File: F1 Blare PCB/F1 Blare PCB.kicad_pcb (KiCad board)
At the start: 2 copper layers, 79 x 58 mm, 11 parts, among them J1 Conn_01x08_Pin, SW1 SW_Push, SW2 SW_Push, SW3 SW_Push, SW4 SW_Push, U1 XIAO-ESP32-C3-SMD

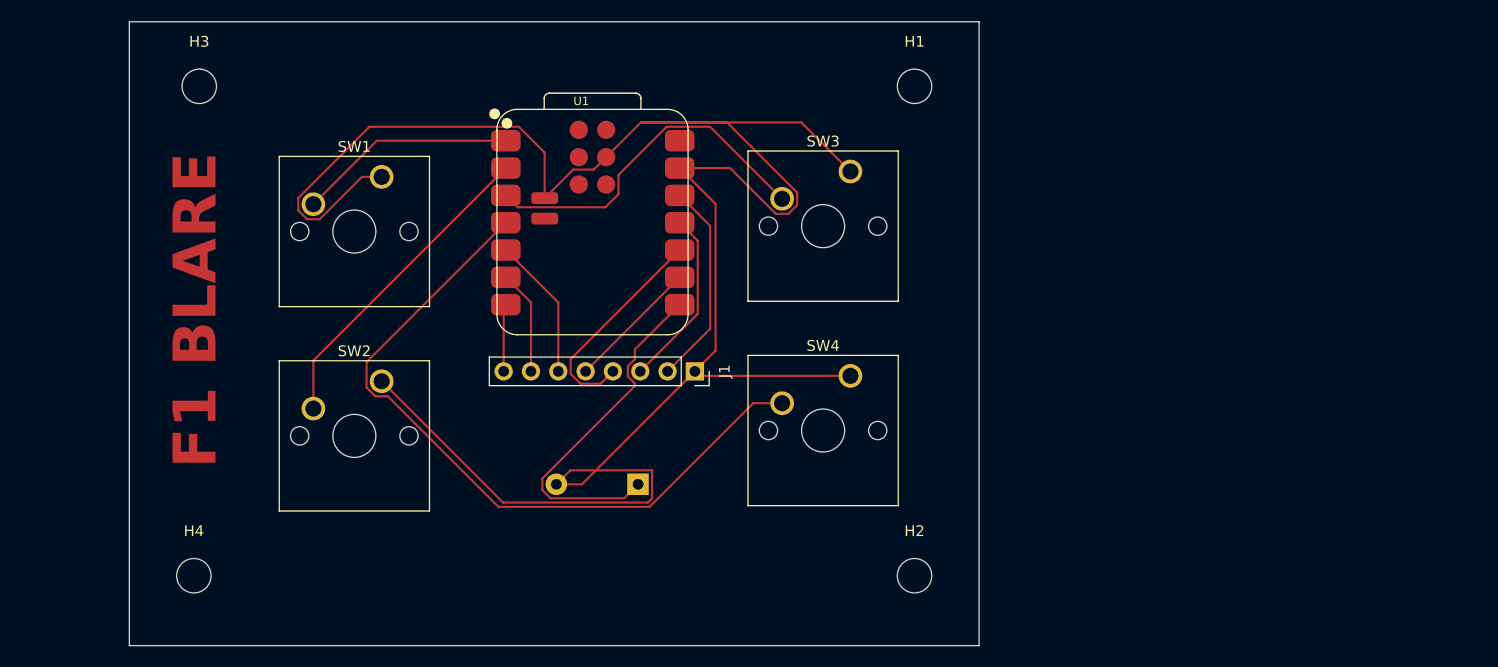
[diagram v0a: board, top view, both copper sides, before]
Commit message: PCB Finalization & CAD Design
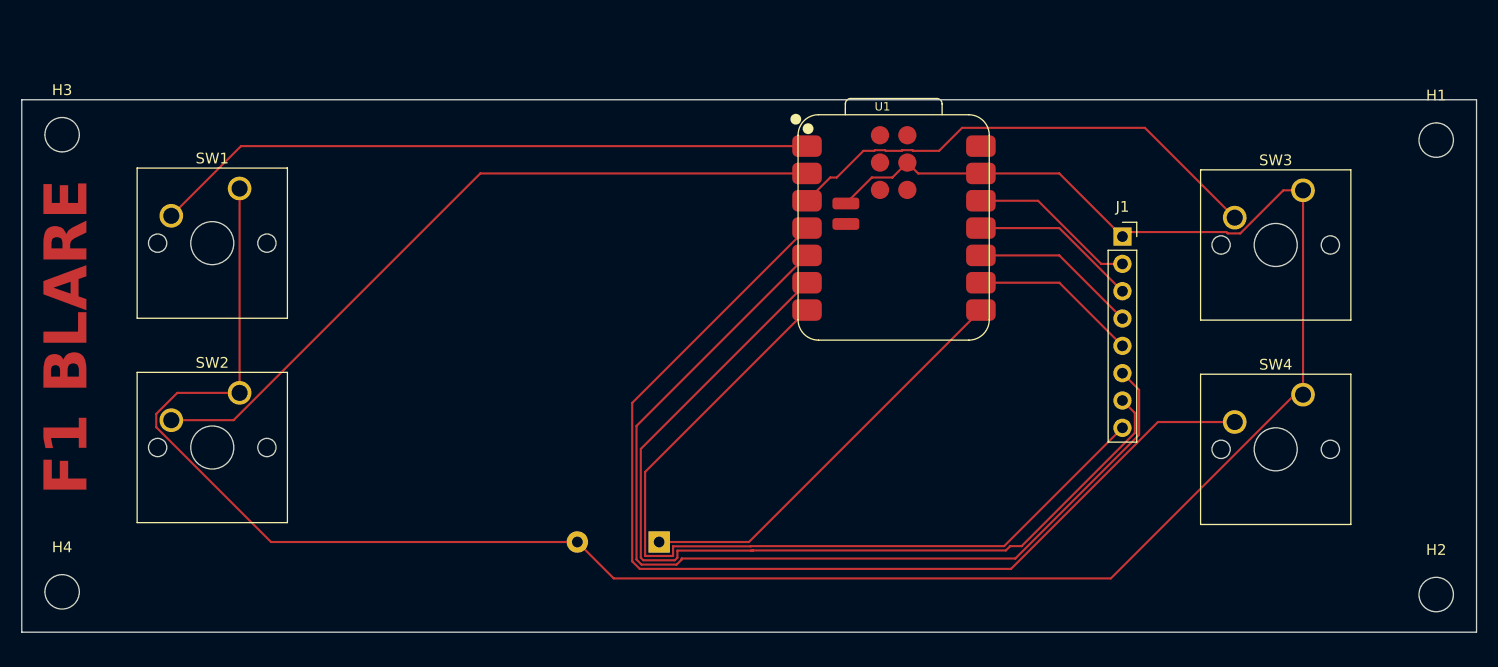
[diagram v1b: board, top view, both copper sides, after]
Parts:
- moved H1 48.8 mm to (219.0, 90.0)
- moved H2 48.5 mm to (219.0, 132.2)
- moved SW3 42.1 mm to (206.6, 94.7)
- moved SW4 42.1 mm to (206.6, 113.7)
- moved J1 41.7 mm to (189.8, 99.0), turned to 0 degrees
- moved U1 28.0 mm to (159.7, 108.7)
- moved H3 13.5 mm to (91.2, 89.5)
- moved SW1 13.3 mm to (107.8, 94.5)
- moved SW2 13.3 mm to (107.8, 113.5)
- moved H4 12.3 mm to (91.2, 132.0)
- moved BZ1 5.71 mm to (146.8, 127.4)
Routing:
- net /DC: track 13.3 -> 93.2 mm
- net /CS: track 9.71 -> 86.8 mm
- net /BL: track 6.28 -> 78.9 mm
- net Net-(U1-D0): track 20.3 -> 61.8 mm
- net Net-(U1-D1): track 29.8 -> 68.6 mm
- net Net-(U1-D3): track 67.9 -> 99.7 mm
- net GND: track 201.4 -> 217.1 mm
- net Net-(U1-D2): track 33.1 -> 46.1 mm
- net Net-(BZ1-+): track 32.8 -> 38.8 mm
- net /SCL: track 20.8 -> 15.6 mm
- net +3V3: track 19.9 -> 15.6 mm
- net /RST: track 12.4 -> 15.6 mm
- net /SDA: track 16.7 -> 15.6 mm
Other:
- board size 79 x 58 mm -> 135.2 x 49.5 mm
